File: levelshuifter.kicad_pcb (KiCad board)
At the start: 2 copper layers, 57 x 117 mm, 25 parts, among them J1 Screw_Terminal_01x02, J2 Conn_02x20_Odd_Even, J3 Conn_02x08_Odd_Even, J4 Conn_02x08_Odd_Even, J5 Conn_02x08_Odd_Even, U1 LM1117-3.3, U2 74LVC8T245PW, U3 74LVC8T245PW, U4 74LVC8T245PW, U5 L7805, U6 74LVC8T245PW, U7 74LVC8T245PW

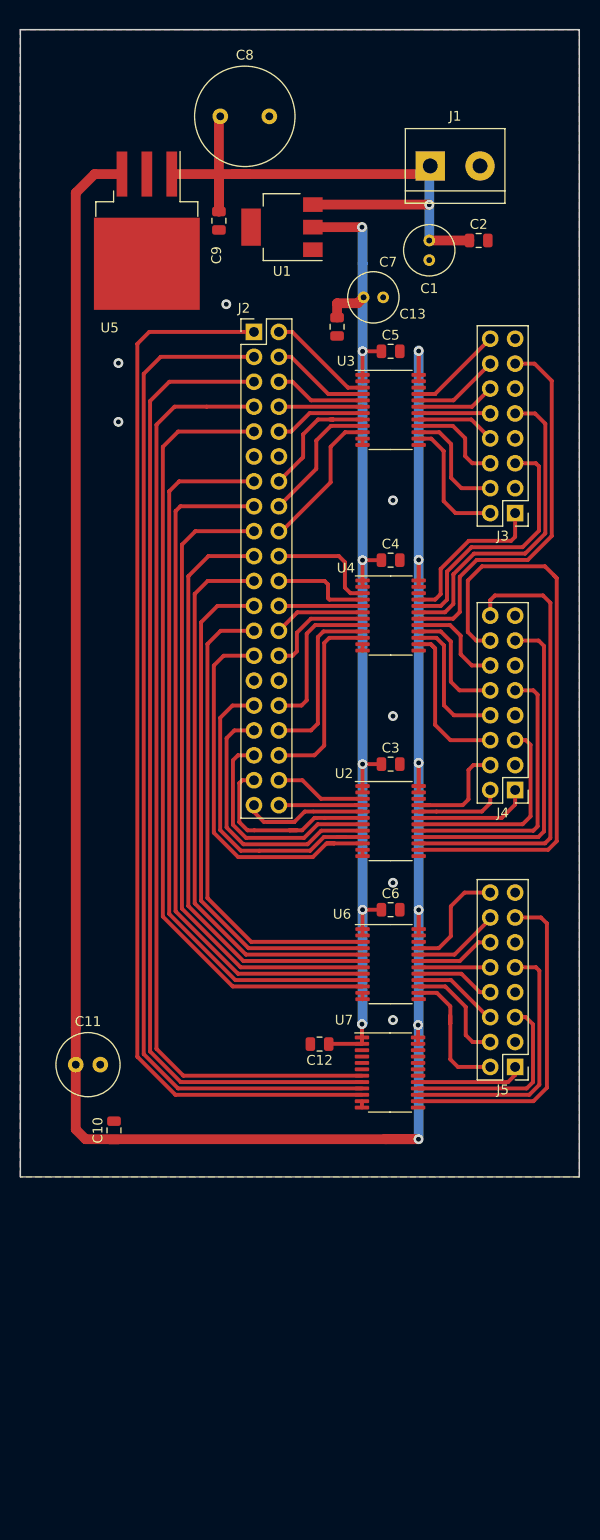
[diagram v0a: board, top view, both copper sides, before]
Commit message: segundos cambios
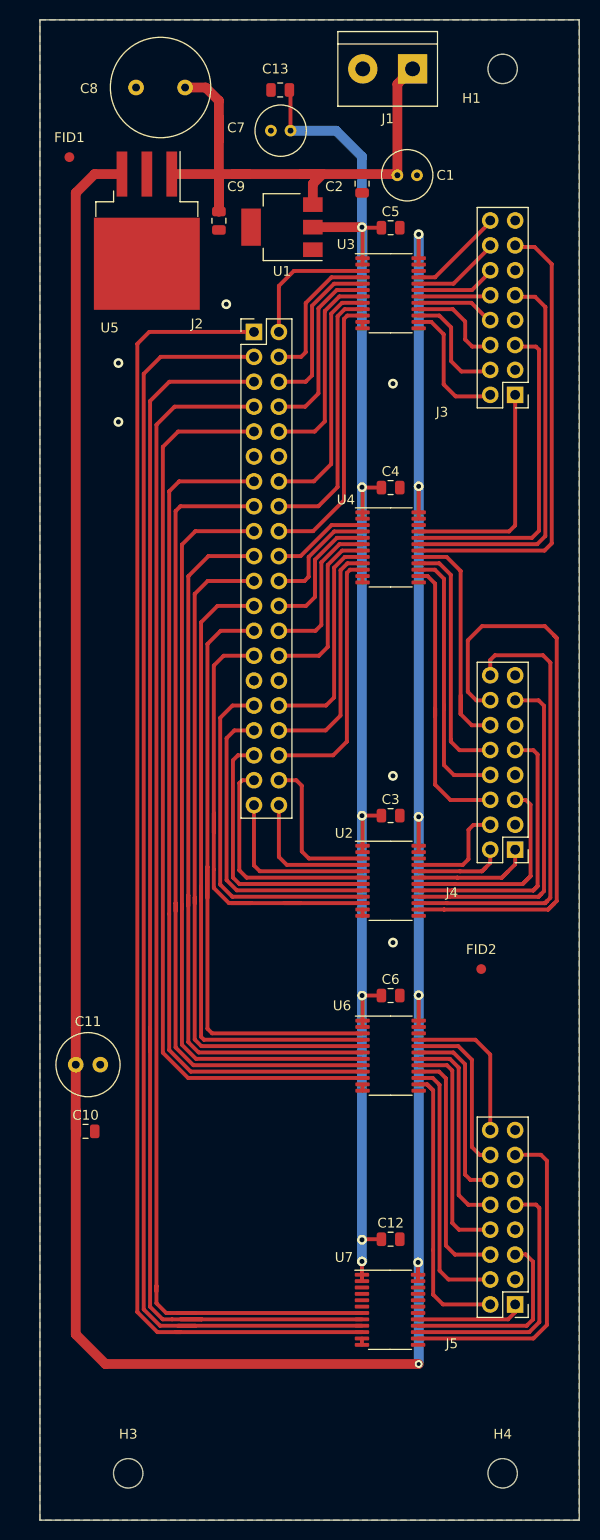
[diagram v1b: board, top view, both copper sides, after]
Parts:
- added FID1: Fiducial, Fiducial:Fiducial_1mm_Mask2mm, F.Cu at (60.0, 42.0)
- added FID2: Fiducial, Fiducial:Fiducial_1mm_Mask2mm, F.Cu at (102.0, 124.8)
- added H1: MountingHole, MountingHole:MountingHole_3mm, F.Cu at (104.2, 33.0)
- added H3: MountingHole, MountingHole:MountingHole_3mm, F.Cu at (66.0, 176.2)
- added H4: MountingHole, MountingHole:MountingHole_3mm, F.Cu at (104.2, 176.2)
- C10: value 1uF -> 4.7uF
- moved C13 24.8 mm to (81.5, 35.1), turned to 180 degrees
- moved J5 24.2 mm to (105.5, 159.0)
- moved U7 24.2 mm to (92.7, 159.6)
- moved C12 21.2 mm to (92.8, 152.3), turned to 0 degrees
- moved C7 18.6 mm to (82.5, 39.3), turned to 180 degrees
- moved C2 13.2 mm to (89.8, 44.7), turned to 270 degrees
- moved C5 12.6 mm to (92.8, 49.2)
- moved J3 12.1 mm to (105.5, 66.2)
- moved U3 11.9 mm to (92.8, 55.9)
- moved J1 10.1 mm to (95.0, 33.0), turned to 180 degrees
- moved U6 9.33 mm to (92.8, 133.6)
- moved C6 8.75 mm to (92.8, 127.5)
- moved C1 7.40 mm to (93.5, 43.9), turned to 0 degrees
- moved C4 7.40 mm to (92.8, 75.7)
- moved U4 6.95 mm to (92.8, 81.8)
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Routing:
- net +5V: track 233.2 -> 290.5 mm
- net +3V3: track 127.6 -> 163.1 mm
- net /A5_6: track 100.6 -> 130.5 mm
- net /A5_5: track 96.4 -> 123.8 mm
- net /A5_7: track 105.0 -> 132.1 mm
- net /A5_8: track 109.6 -> 135.4 mm
- net Net-(J5-Pad6): track 8.86 -> 25.2 mm
- net Net-(J5-Pad4): track 11.5 -> 27.1 mm
- net Net-(J5-Pad8): track 8.08 -> 23.4 mm
- net Net-(J5-Pad2): track 14.4 -> 29.7 mm
- net /A4_1: track 48.9 -> 63.7 mm
- net Net-(J4-Pad12): track 10.1 -> 24.9 mm
- net /A1_8: track 14.8 -> 28.8 mm
- net Net-(J5-Pad10): track 7.30 -> 21.1 mm
- net /A4_2: track 53.0 -> 66.4 mm
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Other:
- board size 57 x 117 mm -> 55 x 153 mm
